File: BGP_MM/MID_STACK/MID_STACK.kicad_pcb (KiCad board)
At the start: 2 copper layers, 26 x 28 mm, 13 parts, among them J1 Conn_01x04_Male, J2 Conn_01x02_Male, J3 Conn_01x04_Male, J4 Conn_01x04_Male, P1 CONN_01X09, P2 CONN_01X02, P3 CONN_01X02, P4 CONN_01X03

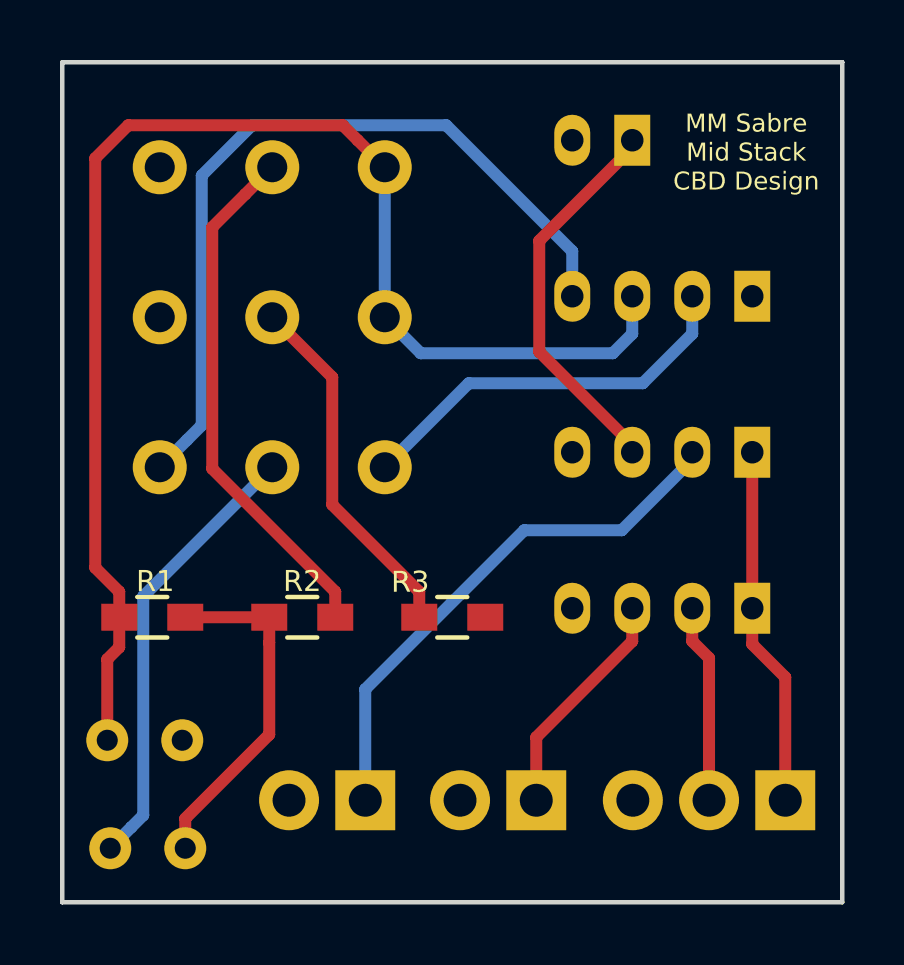
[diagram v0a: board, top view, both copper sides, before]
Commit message: MM - Board changes
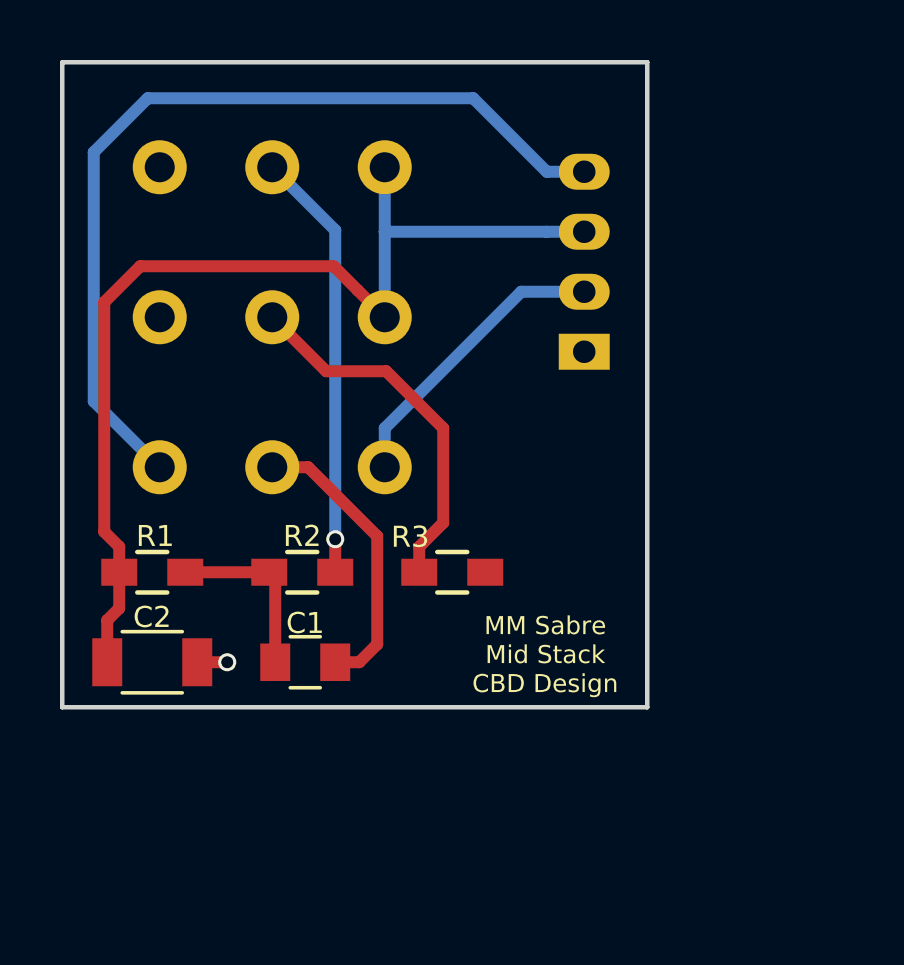
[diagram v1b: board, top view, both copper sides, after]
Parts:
- removed J2: Conn_01x02_Male, Connectors_JST:JST_PH_B2B-PH-K_02x2.00mm_Straight
- removed J3, J4: Conn_01x04_Male, Connectors_JST:JST_PH_B4B-PH-K_04x2.00mm_Straight
- removed P2, P3: CONN_01X02, Terminal_Blocks:TerminalBlock_Pheonix_MPT-2.54mm_2pol
- removed P4: CONN_01X03, Terminal_Blocks:TerminalBlock_Pheonix_MPT-2.54mm_3pol
- C1: footprint Capacitor_THT:C_Rect_L4.6mm_W3.0mm_P2.50mm_MKS02_FKP02 -> Capacitors_SMD:C_0805; moved to F.Cu
- C2: footprint Capacitor_THT:C_Rect_L4.6mm_W3.0mm_P2.50mm_MKS02_FKP02 -> Capacitors_SMD:C_1206; moved to F.Cu
- moved C1 8.98 mm to (137.1, 101.0), turned to 180 degrees
- moved J1 5.90 mm to (146.4, 90.7), turned to 90 degrees
- moved C2 3.00 mm to (132.0, 101.0)
- moved R1 1.50 mm to (132.0, 98.0)
- moved R2 1.50 mm to (137.0, 98.0)
- moved R3 1.50 mm to (142.0, 98.0)
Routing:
- net /JZ_I: track 18.0 -> 0.00 mm
- net /SIG_O: track 13.0 -> 0.00 mm
- net /MM_BH: track 12.1 -> 0.00 mm
- net /MID_R: track 45.8 -> 34.6 mm
- net /MM_NH: track 7.73 -> 0.00 mm
- net /MM_BC: track 6.63 -> 0.00 mm
- net Net-(C1-Pad2): track 11.7 -> 5.88 mm
- net /VOL2: track 14.9 -> 9.70 mm
- net /MID_O: track 13.3 -> 9.83 mm
- net /F1_2: track 17.5 -> 14.4 mm, vias 0 -> 1
- net /MID_I: track 26.6 -> 29.5 mm
- net /Vref: track 0.00 -> 1.00 mm, vias 0 -> 1
- added copper zone on B.Cu, net /Vref
- removed copper zone on B.Cu, net Earth
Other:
- board size 26 x 28 mm -> 19.5 x 21.5 mm
